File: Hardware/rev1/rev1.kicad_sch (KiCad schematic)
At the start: 0 parts

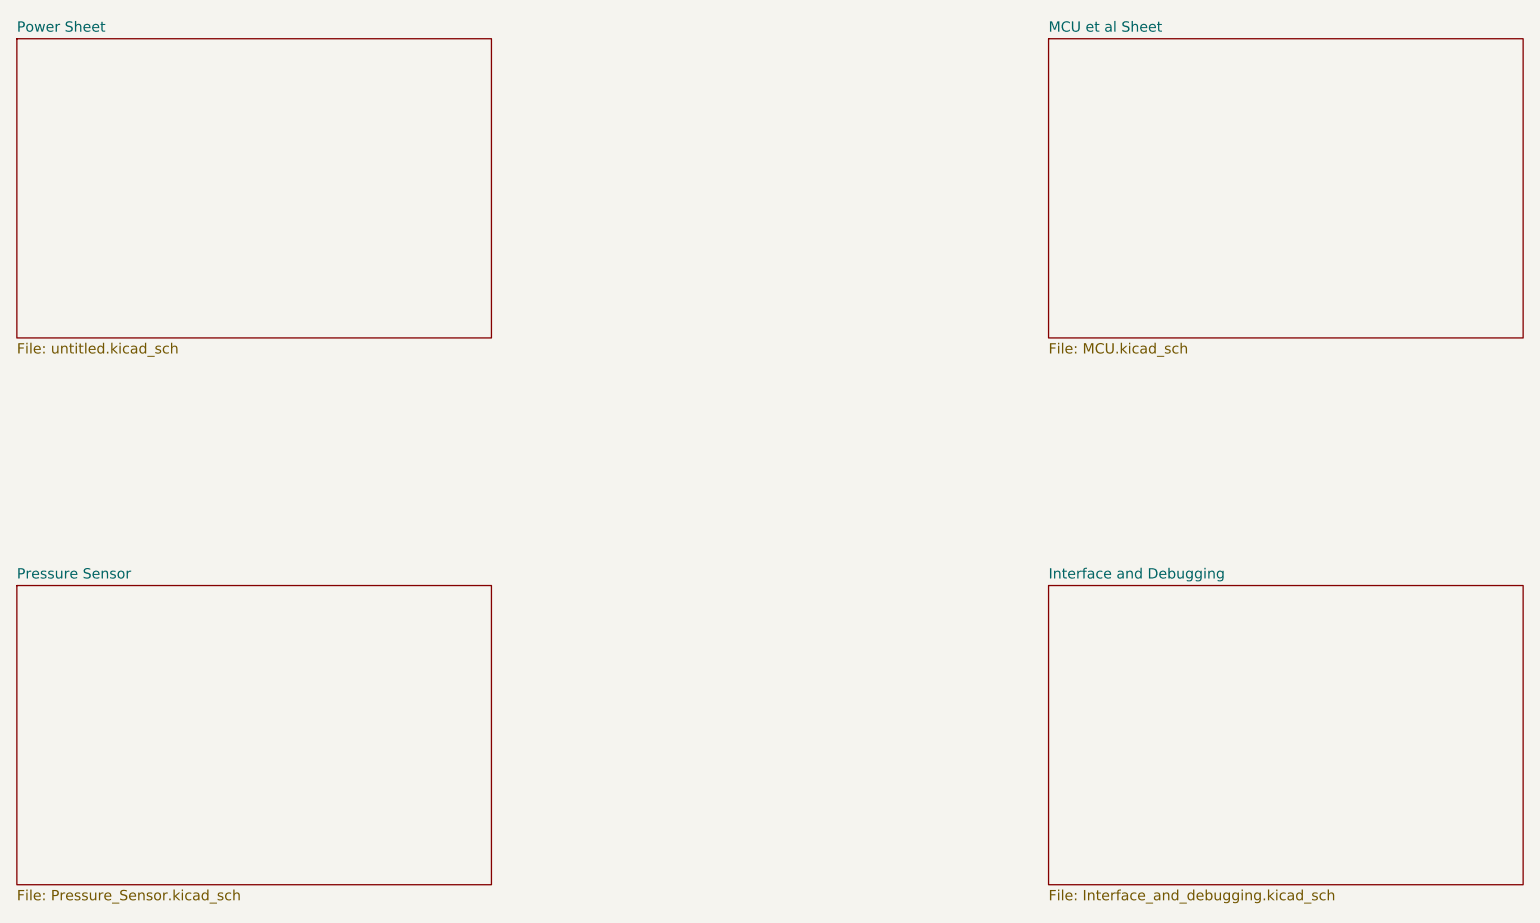
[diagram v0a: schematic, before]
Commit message: h
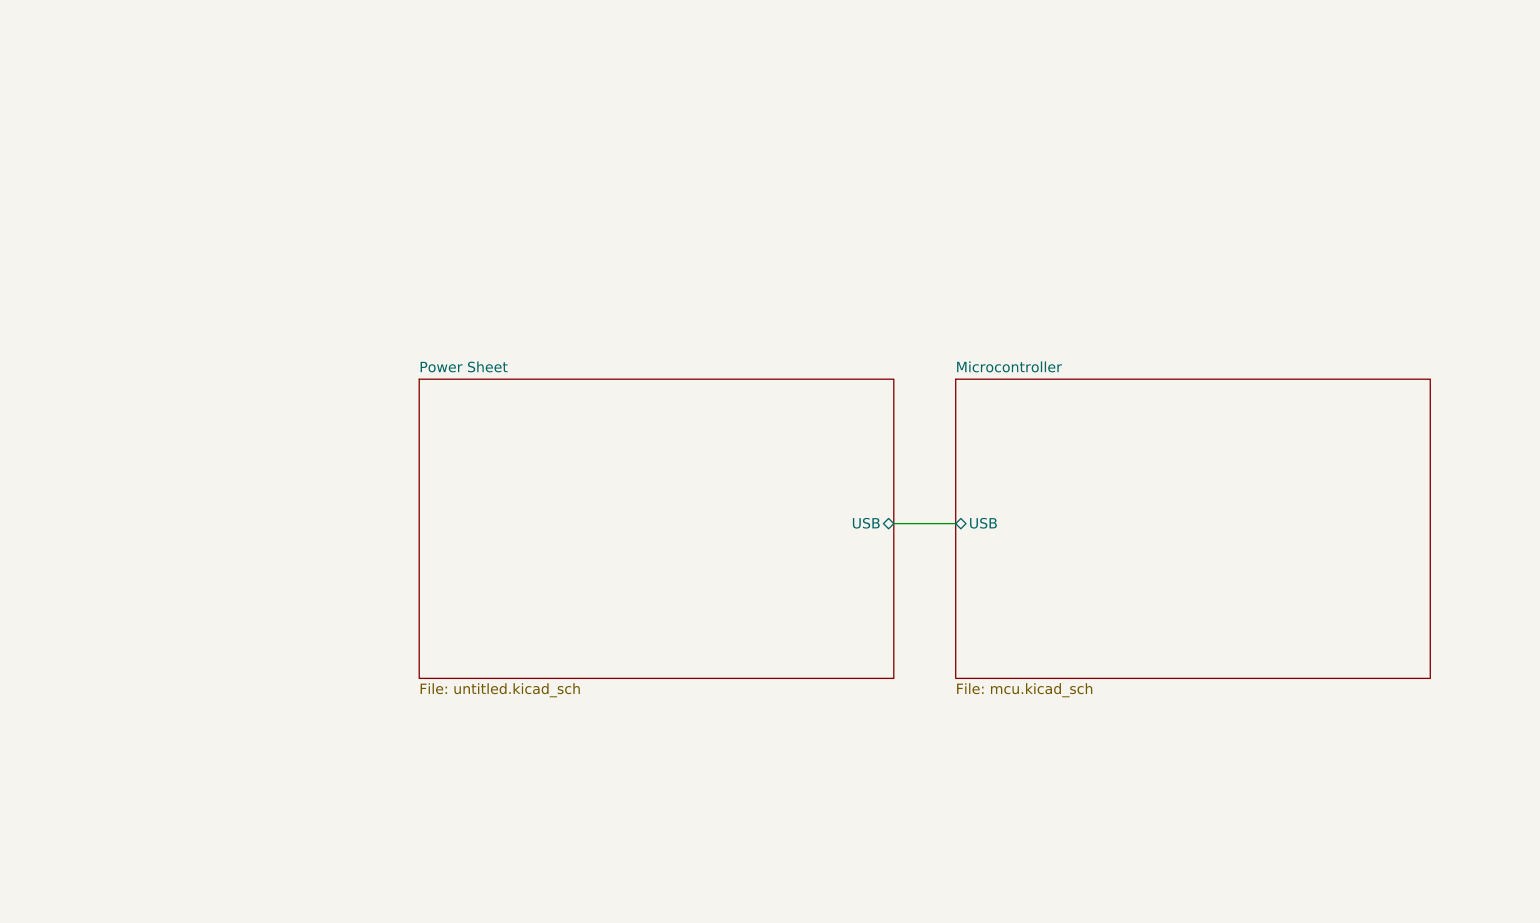
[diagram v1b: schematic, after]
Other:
- removed sheet Interface and Debugging
- removed sheet MCU et al Sheet
- removed sheet Pressure Sensor
- added sheet Microcontroller (mcu.kicad_sch)
- sheet Power Sheet ports: added USB; removed none
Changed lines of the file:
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@@
 		(company "StrathGREM Ltd.")
 	)
+	(wire
+		(pts
+			(xy 144.78 95.25) (xy 152.4 95.25)
+		)
+		(stroke
+			(width 0)
+			(type default)
+		)
+	)
 	(sheet
-		(at 36.83 102.87)
+		(at 152.4 77.47)
 		(size 58.42 36.83)
 		(fields_autoplaced yes)
@@
 			(color 0 0 0 0.0000)
 		)
-		(property "Sheetname" "Pressure Sensor"
-			(at 36.83 102.1584 0)
+		(property "Sheetname" "Microcontroller"
+			(at 152.4 76.7584 0)
 			(effects
 				(font
@@
 			)
 		)
-		(property "Sheetfile" "Pressure_Sensor.kicad_sch"
-			(at 36.83 140.2846 0)
+		(property "Sheetfile" "mcu.kicad_sch"
+			(at 152.4 114.8846 0)
 			(effects
 				(font
@@
 				)
 				(justify left top)
+			)
+		)
+		(pin "USB" bidirectional
+			(at 152.4 95.25 180)
+			(effects
+				(font
+					(size 1.27 1.27)
+				)
+				(justify left)
 			)
 		)
@@
 	)
 	(sheet
-		(at 36.83 35.56)
+		(at 86.36 77.47)
 		(size 58.42 36.83)
 		(fields_autoplaced yes)
@@
 		)
 		(property "Sheetname" "Power Sheet"
-			(at 36.83 34.8484 0)
+			(at 86.36 76.7584 0)
 			(effects
 				(font
@@
 		)
 		(property "Sheetfile" "untitled.kicad_sch"
-			(at 36.83 72.9746 0)
+			(at 86.36 114.8846 0)
 			(effects
 				(font
@@
 				)
 				(justify left top)
+			)
+		)
+		(pin "USB" bidirectional
+			(at 144.78 95.25 0)
+			(effects
+				(font
+					(size 1.27 1.27)
+				)
+				(justify right)
 			)
 		)
@@
 				)
 			)
-		)
-	)
-	(sheet
-		(at 163.83 102.87)
-		(size 58.42 36.83)
-		(fields_autoplaced yes)
-		(stroke
-			(width 0.1524)
-			(type solid)
-		)
-		(fill
-			(color 0 0 0 0.0000)
-		)
-		(property "Sheetname" "Interface and Debugging"
-			(at 163.83 102.1584 0)
-			(effects
-				(font
-					(size 1.27 1.27)
-				)
-				(justify left bottom)
-			)
-		)
-		(property "Sheetfile" "Interface_and_debugging.kicad_sch"
-			(at 163.83 140.2846 0)
-			(effects
-				(font
-					(size 1.27 1.27)
-				)
-				(justify left top)
-			)
-		)
-		(instances
-			(project "rev1"
-				(path "/e52639ab-1647-4d34-8bc5-5aadc4708147"
-					(page "4")
-				)
-			)
-		)
-	)
-	(sheet
-		(at 163.83 35.56)
-		(size 58.42 36.83)
-		(fields_autoplaced yes)
-		(stroke
-			(width 0.1524)
-			(type solid)
-		)
-		(fill
-			(color 0 0 0 0.0000)
-		)
-		(property "Sheetname" "MCU et al Sheet"
-			(at 163.83 34.8484 0)
-			(effects
-				(font
-					(size 1.27 1.27)
-				)
-				(justify left bottom)
-			)
-		)
-		(property "Sheetfile" "MCU.kicad_sch"
-			(at 163.83 72.9746 0)
-			(effects
-				(font
-					(size 1.27 1.27)
-				)
-				(justify left top)
-			)
-		)
-		(instances
-			(project "rev1"
-				(path "/e52639ab-1647-4d34-8bc5-5aadc4708147"
-					(page "3")
-				)
-			)
